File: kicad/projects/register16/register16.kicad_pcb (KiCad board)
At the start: 2 copper layers, 42 parts, among them J1 INPUT_ENABLE, J10 LOW, J2 OUTPUT_ENABLE, J3 CONTENTS, J4 Control_signal_backplane, J5 Aux_connection, J6 Bus_connection, J7 HIGH, J8 LOW, J9 HIGH, U1 74HCT04, U2 74HCT377, U3 74HCT377, U4 74HCT245, U5 74HCT245, U6 74HCT245, U7 74HCT245

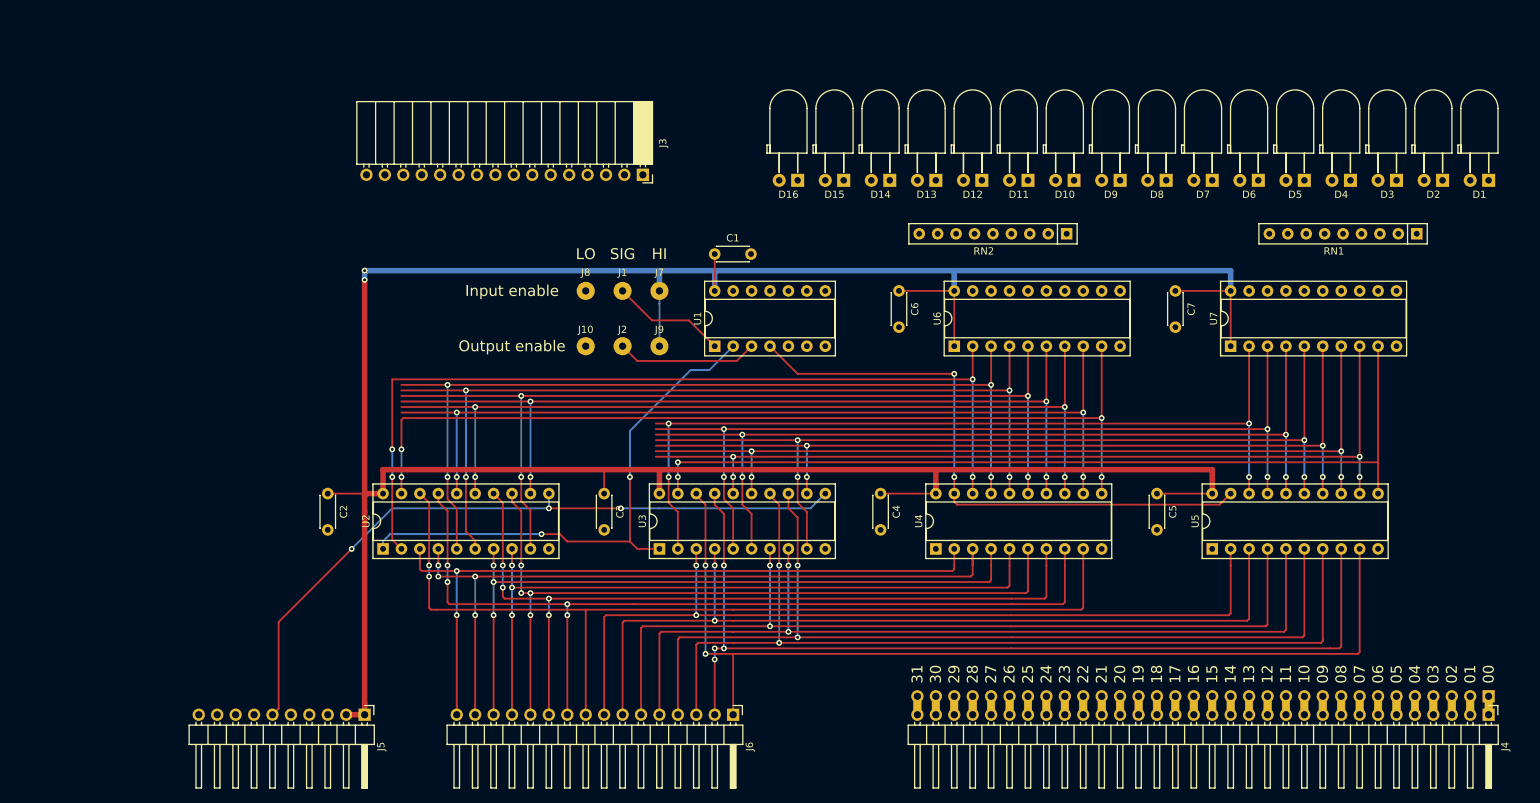
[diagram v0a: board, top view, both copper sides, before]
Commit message: Register mostly complete
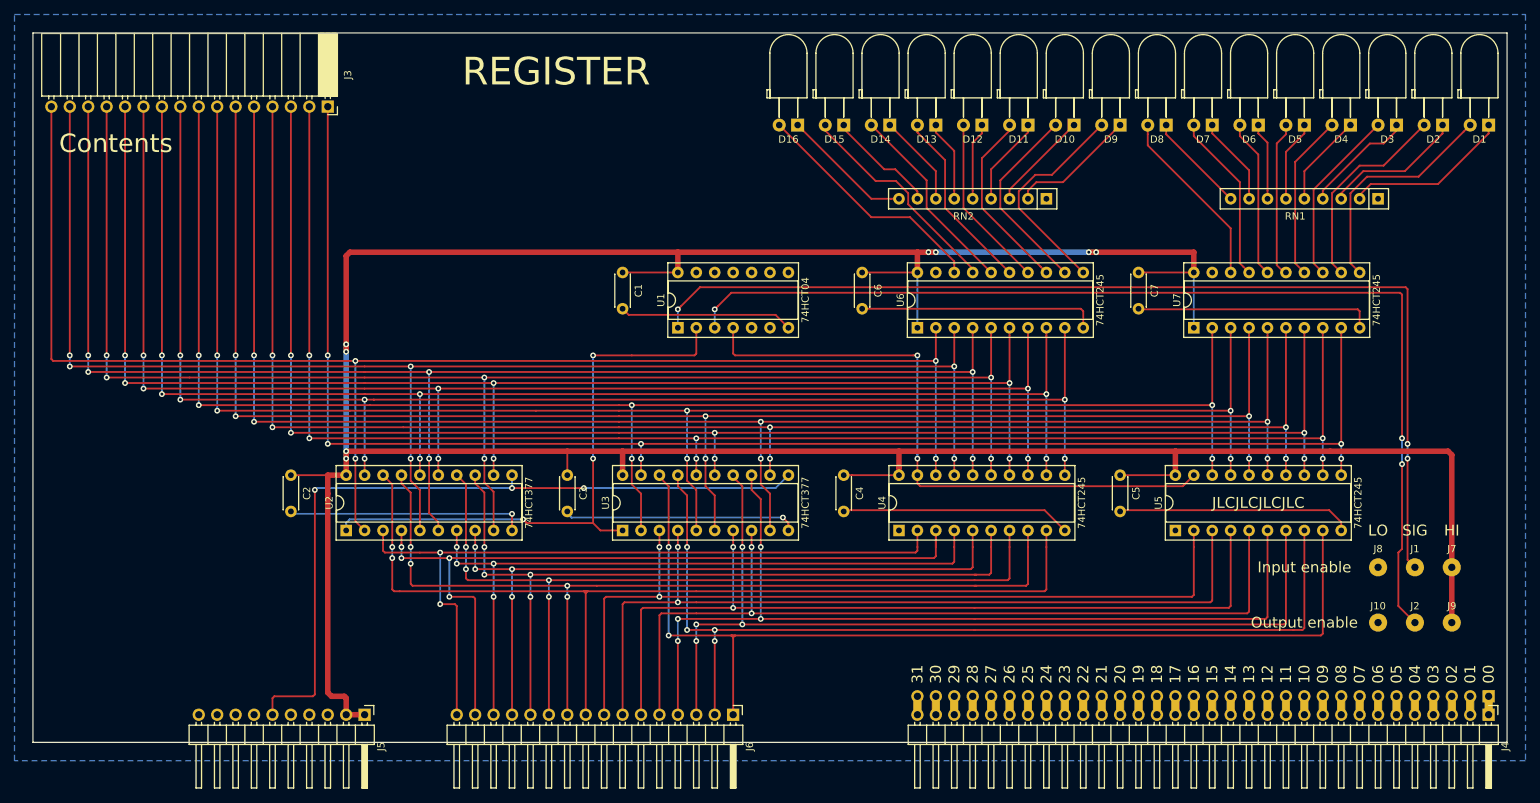
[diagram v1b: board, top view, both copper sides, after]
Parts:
- D1, D10, D11, D12, D13, D14, D15, D16, D2, D3, D4, D5, D6, D7, D8, D9: footprint LED_THT:LED_D5.0mm_Horizontal_O3.81mm_Z3.0mm -> eight-bit-computer:LED_D5.0mm_Horizontal_O3.81mm_Z3.0mm
- moved J1 115.7 mm to (264.2, 111.8)
- moved J2 115.7 mm to (264.2, 119.4)
- moved J7 115.7 mm to (269.2, 111.8)
- moved J8 115.7 mm to (259.1, 111.8)
- moved J9 115.7 mm to (269.2, 119.4)
- moved J10 115.7 mm to (259.1, 119.4)
- moved J3 44.4 mm to (114.3, 48.3)
- moved C1 13.0 mm to (154.9, 71.1), turned to 270 degrees
- moved D1 7.62 mm to (274.3, 50.8)
- moved D10 7.62 mm to (217.2, 50.8)
- moved D11 7.62 mm to (210.8, 50.8)
- moved D12 7.62 mm to (204.5, 50.8)
- moved D13 7.62 mm to (198.1, 50.8)
- moved D14 7.62 mm to (191.8, 50.8)
- moved D15 7.62 mm to (185.4, 50.8)
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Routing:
- net GND: track 0.00 -> 218.9 mm, vias 0 -> 2
- net Net-(J1-Pad1): track 15.9 -> 143.3 mm, vias 0 -> 3
- net Net-(J2-Pad1): track 19.5 -> 144.7 mm, vias 0 -> 3
- net /CNT07: track 119.9 -> 219.0 mm, vias 4 -> 6
- net /CNT06: track 122.2 -> 220.0 mm, vias 4 -> 6
- net /CNT05: track 124.0 -> 219.5 mm, vias 4 -> 6
- net /CNT04: track 125.5 -> 219.2 mm, vias 4 -> 6
- net /CNT03: track 119.4 -> 211.3 mm, vias 4 -> 6
- net /CNT02: track 121.2 -> 211.3 mm, vias 4 -> 6
- net /CNT00: track 121.4 -> 211.3 mm, vias 2 -> 6
- net /CNT01: track 122.9 -> 211.3 mm, vias 4 -> 6
- net /CNT15: track 124.2 -> 201.0 mm
- net /CNT14: track 124.8 -> 201.5 mm, vias 4 -> 6
- net /CNT13: track 126.5 -> 201.2 mm, vias 4 -> 6
- net /CNT12: track 128.3 -> 201.2 mm, vias 4 -> 6
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- added copper zone on B.Cu, net GND
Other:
- board outline added: 203.2 x 97.8 mm
- net class Default: clearance 0.1778 -> 0.2
- rule trace_clearance: 0.1778 -> 0.2
- board text added: "Contents"
- board text added: "JLCJLCJLCJLC"
- board text added: "REGISTER"
